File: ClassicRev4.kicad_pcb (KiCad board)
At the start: 2 copper layers, 65 x 50 mm, 65 parts, among them IC1 7805TV, IC2 MEGA8-P, IC3 K155ID1, Q1 IRF740, Q2 16MHz, Q3 2N7000, Q4 2N7000, Q5 2N7000, Q6 2N7000

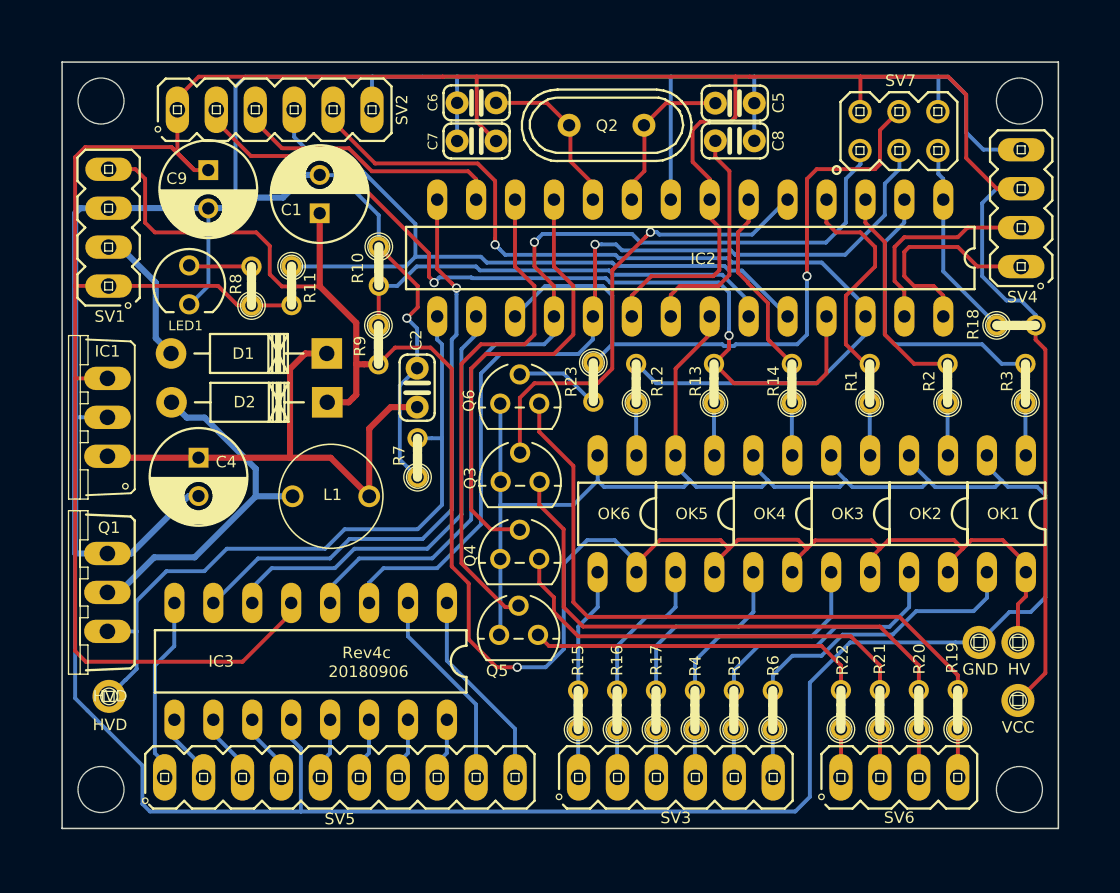
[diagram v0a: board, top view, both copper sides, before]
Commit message: KiCad 5
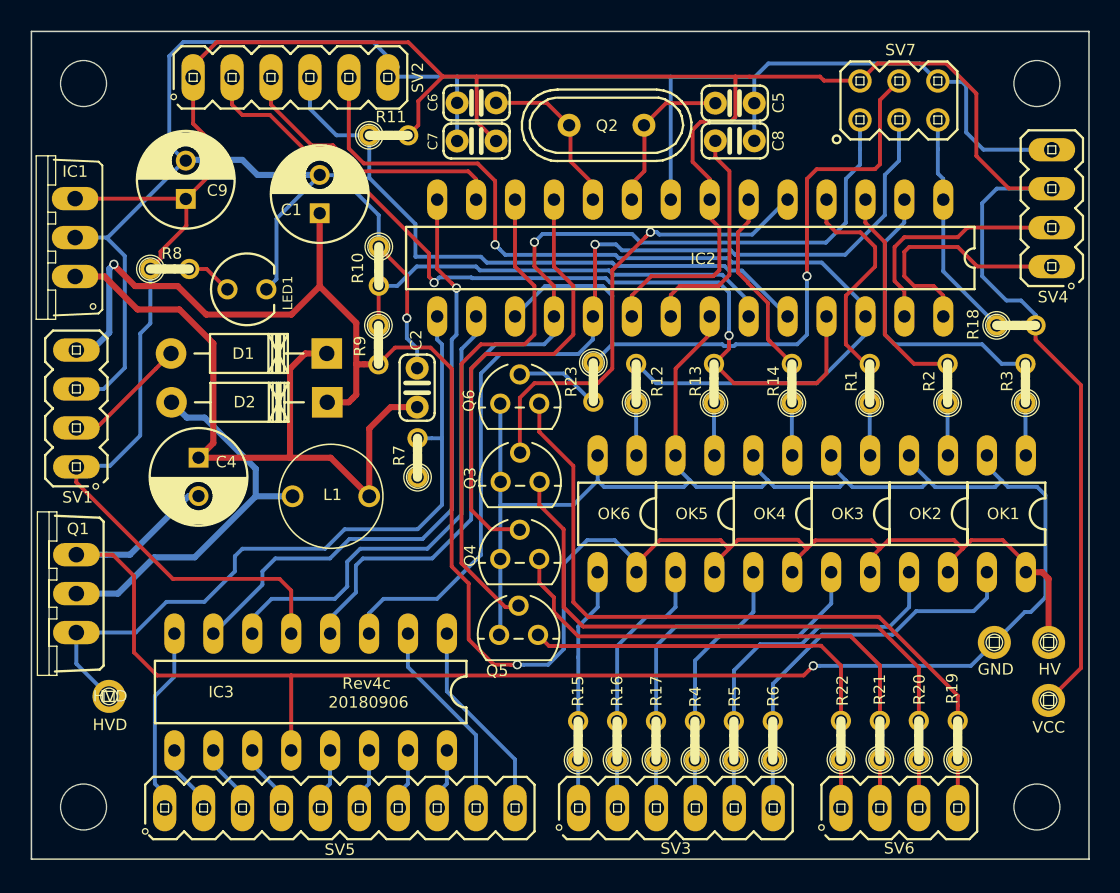
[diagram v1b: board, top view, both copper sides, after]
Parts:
- moved SV1 12.0 mm to (118.8, 112.3)
- moved IC1 11.9 mm to (116.2, 101.1)
- moved R11 11.7 mm to (139.2, 94.5), turned to 0 degrees
- moved R8 5.44 mm to (124.9, 103.2), turned to 0 degrees
- moved LED1 3.78 mm to (129.9, 104.5), turned to 0 degrees
- moved C9 2.39 mm to (125.9, 98.6), turned to 90 degrees
- moved SV2 2.35 mm to (132.8, 90.7)
- moved Q1 2.03 mm to (116.3, 124.4)
- moved IC3 2.00 mm to (134.1, 130.8)
- moved R15 2.00 mm to (151.5, 134.0)
- moved R16 2.00 mm to (154.1, 134.0)
- moved R17 2.00 mm to (156.6, 134.0)
- moved R19 2.00 mm to (176.3, 133.9)
- moved R20 2.00 mm to (173.8, 133.9)
- moved R21 2.00 mm to (171.2, 133.9)
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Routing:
- net GND: track 341.0 -> 312.7 mm, vias 1 -> 2
- net /VCC: track 211.9 -> 198.5 mm
- net /VIN: track 34.9 -> 47.6 mm
- net /DLS: track 48.4 -> 41.7 mm
- net /DIGIT_A: track 60.0 -> 64.0 mm
- net /DIGIT_D: track 61.3 -> 65.0 mm
- net /170V: track 122.5 -> 125.6 mm, vias 1 -> 2
- net /ANODE6: track 61.6 -> 63.7 mm
- net /DRAIN: track 23.8 -> 25.9 mm
- net Net-(Q5-Pad1): track 22.1 -> 24.1 mm
- net /SCL: track 14.3 -> 16.3 mm
- net /SDA: track 13.6 -> 15.6 mm
- net Net-(Q4-Pad1): track 28.2 -> 30.2 mm
- net Net-(OK6-Pad3): track 8.15 -> 10.1 mm
- net Net-(OK5-Pad3): track 9.94 -> 11.9 mm
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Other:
- board size 65 x 50 mm -> 69 x 54 mm
